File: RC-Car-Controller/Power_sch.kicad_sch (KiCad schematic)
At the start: 19 parts, among them U2 A6986F3V3TR, U3 LT1963AxST-3.3

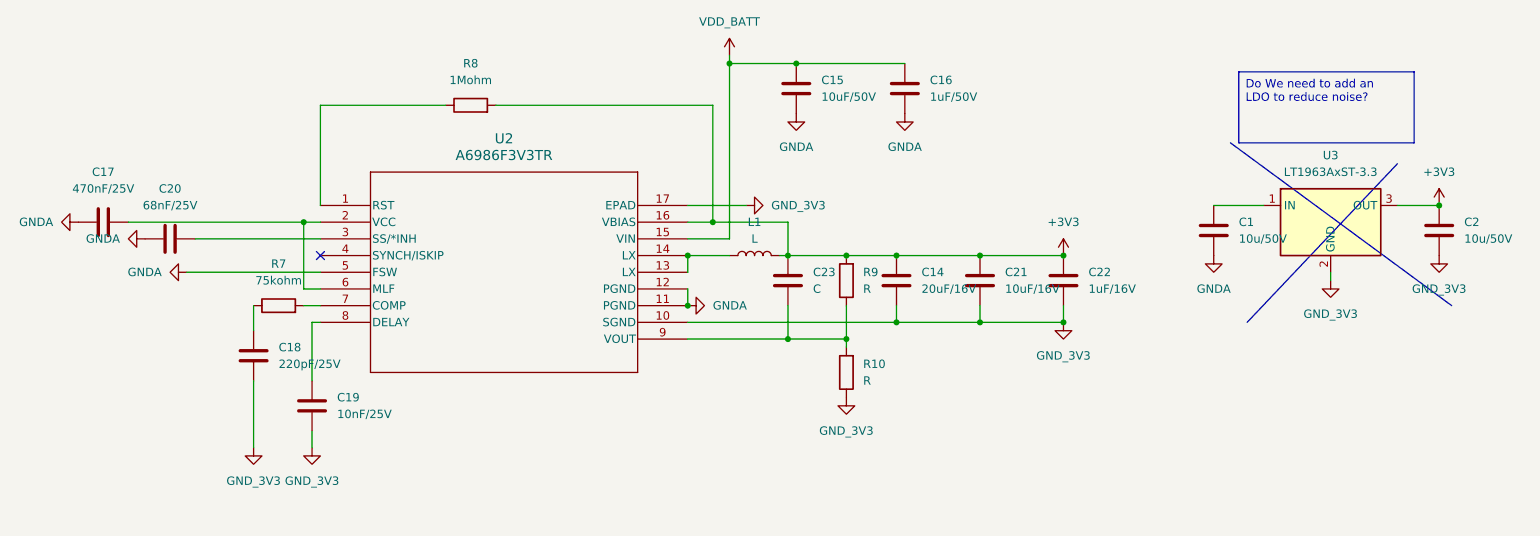
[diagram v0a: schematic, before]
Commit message: Fixed Controller PCB
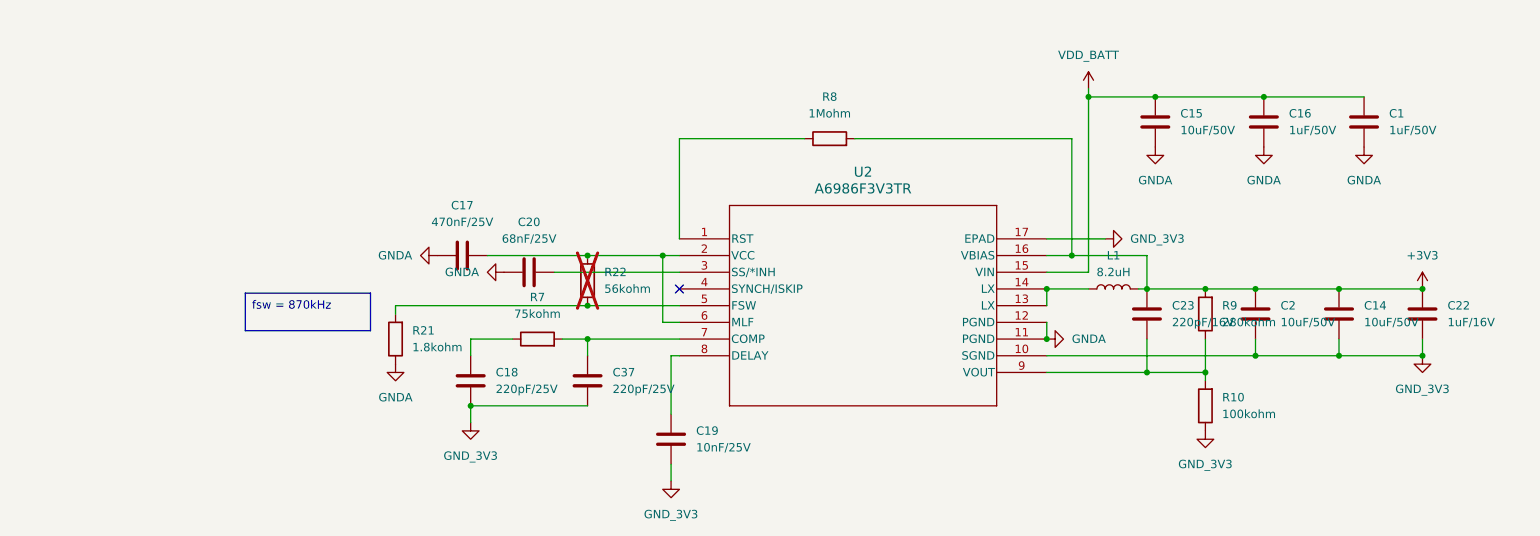
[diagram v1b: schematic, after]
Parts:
- removed C21: 10uF/16V, symbol Device:C
- removed U3: LT1963AxST-3.3, Package_TO_SOT_SMD:SOT-223-3_TabPin2, symbol Regulator_Linear:LT1963AxST-3.3
- added C37: 220pF/25V, Capacitor_SMD:C_0201_0603Metric, symbol Device:C
- added R21: 1.8kohm, Resistor_SMD:R_0201_0603Metric, symbol Device:R
- added R22: 56kohm, Resistor_SMD:R_0201_0603Metric, symbol Device:R
- C1: value 10u/50V -> 1uF/50V; footprint (none) -> Capacitor_SMD:C_0201_0603Metric
- C14: value 20uF/16V -> 10uF/50V; footprint (none) -> Capacitor_SMD:C_1210_3225Metric
- C15: footprint (none) -> Capacitor_SMD:C_1210_3225Metric
- C16, C17, C18, C19, C20, C22: footprint (none) -> Capacitor_SMD:C_0201_0603Metric
- C2: value 10u/50V -> 10uF/50V; footprint (none) -> Capacitor_SMD:C_1210_3225Metric
- C23: value C -> 220pF/16V; footprint (none) -> Capacitor_SMD:C_0201_0603Metric
- L1: value L -> 8.2uH; footprint (none) -> Inductor_SMD:L_Wuerth_MAPI-4030
- R10: value R -> 100kohm; footprint (none) -> Resistor_SMD:R_0201_0603Metric
- R7, R8: footprint (none) -> Resistor_SMD:R_0201_0603Metric
- R9: value R -> 280kohm; footprint (none) -> Resistor_SMD:R_0201_0603Metric
- U2: footprint HTSSOP16_4P5X5P1X0P65P_STM -> footprints:HTSSOP16_4P5X5P1X0P65P_STM
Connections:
- net GNDA: now also R21.1; no longer U2.5 (FSW)
- net GND_3V3: now also C37.1
- net VDD_BATT: now also C1.1
- net at C17.1, U2.2 (VCC), U2.6 (MLF): now also R22.2
- net at R7.2, U2.7 (COMP): now also C37.2
- new net: R21.2, R22.1, U2.5 (FSW)
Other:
- moved on the sheet: C15, C16, C17, C18, C19, C20, C22, C23, L1, R10, R7, R8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
